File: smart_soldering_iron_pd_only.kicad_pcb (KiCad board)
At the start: 2 copper layers, 15 x 99.9 mm, 89 parts, among them J1 Conn_01x04_Pin, J2 TIP_SMALL_END, J3 TIP_MID, U3 ATMEGA328P-AU, U5 CH224K, Y1 16 MHZ

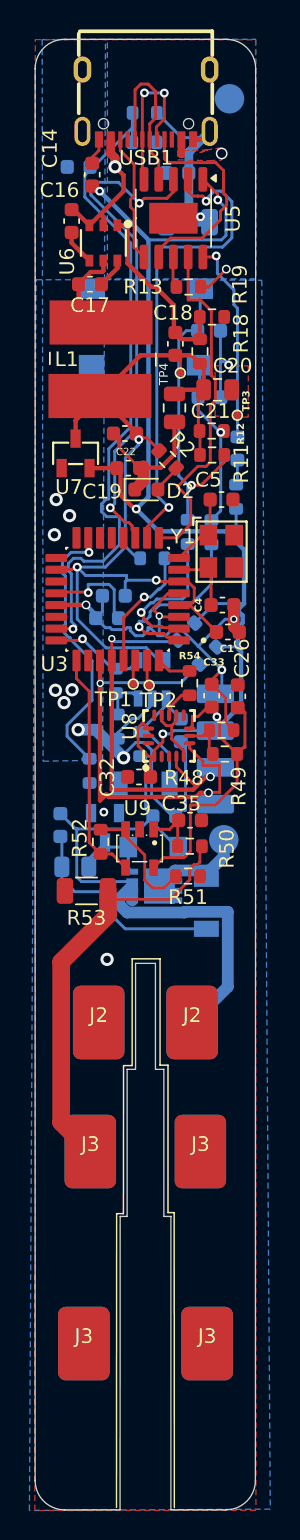
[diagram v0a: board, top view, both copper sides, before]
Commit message: added reset
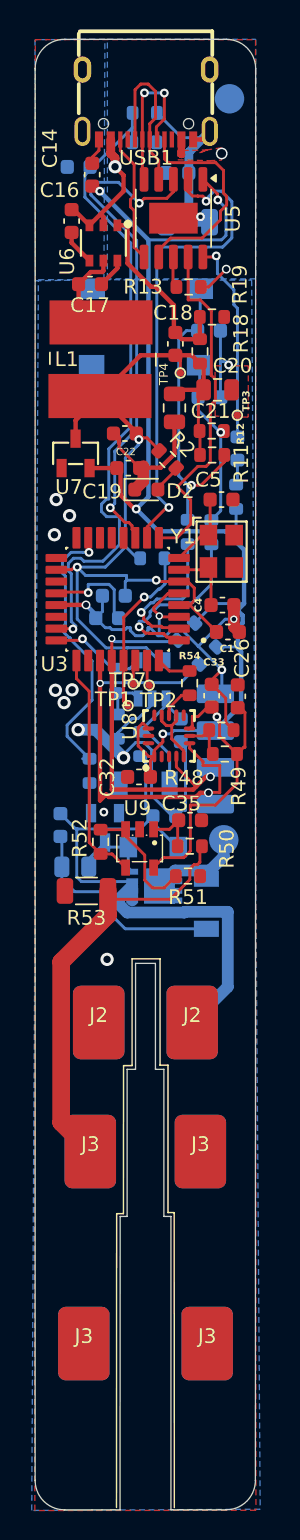
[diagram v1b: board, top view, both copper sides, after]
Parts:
- added TP7: TestPoint, TestPoint:TestPoint_Pad_D1.5mm, F.Cu at (191.3, 95.2)
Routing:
- net Net-(U3-PC6/~{RESET}): track 8.45 -> 11.6 mm
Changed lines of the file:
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@@
 	(footprint "TestPoint:TestPoint_Pad_D1.5mm"
 		(layer "F.Cu")
+		(at 191.3 95.21)
+		(descr "SMD pad as test Point, diameter 1.5mm")
+		(tags "test point SMD pad")
+		(property "Reference" "TP7"
+			(at 0 -1.648 0)
+			(layer "F.SilkS")
+			(effects
+				(font
+					(size 1 1)
+					(thickness 0.15)
+				)
+			)
+		)
+		(property "Value" "TestPoint"
+			(at 0 1.75 0)
+			(layer "F.Fab")
+			(hide yes)
+			(effects
+				(font
+					(size 1 1)
+					(thickness 0.15)
+				)
+			)
+		)
+		(property "Datasheet" "~"
+			(at 0 0 0)
+			(unlocked yes)
+			(layer "F.Fab")
+			(hide yes)
+			(effects
+				(font
+					(size 1.27 1.27)
+					(thickness 0.15)
+				)
+			)
+		)
+		(property "Description" "test point"
+			(at 0 0 0)
+			(unlocked yes)
+			(layer "F.Fab")
+			(hide yes)
+			(effects
+				(font
+					(size 1.27 1.27)
+					(thickness 0.15)
+				)
+			)
+		)
+		(property ki_fp_filters "Pin* Test*")
+		(sheetname "/")
+		(sheetfile "smart_soldering_iron_pd_only.kicad_sch")
+		(attr exclude_from_pos_files)
+		(fp_circle
+			(center 0.01 0.08)
+			(end 0.34 0.06)
+			(stroke
+				(width 0.12)
+				(type solid)
+			)
+			(fill no)
+			(layer "F.SilkS")
+		)
+		(fp_circle
+			(center 0.01 0.08)
+			(end 0.43 0)
+			(stroke
+				(width 0.05)
+				(type solid)
+			)
+			(fill no)
+			(layer "F.CrtYd")
+		)
+		(pad "1" smd circle
+			(at 0.01 0.08)
+			(size 0.5 0.5)
+			(layers "F.Cu" "F.Mask")
+			(net 62 "Net-(U3-PC6{slash}~{RESET})")
+			(pinfunction "1")
+			(pintype "passive")
+		)
+		(embedded_fonts no)
+	)
+	(footprint "TestPoint:TestPoint_Pad_D1.5mm"
+		(layer "F.Cu")
 		(at 191.66 93.74)
 		(descr "SMD pad as test Point, diameter 1.5mm")
@@
 	)
 	(segment
+		(start 191.01 92.22)
+		(end 191.01 94.99)
+		(width 0.2)
+		(layer "F.Cu")
+		(net 62)
+	)
+	(segment
 		(start 192.41 87.9)
 		(end 191.02 89.29)
@@
 	)
 	(segment
+		(start 191.01 94.99)
+		(end 191.31 95.29)
+		(width 0.2)
+		(layer "F.Cu")
+		(net 62)
+	)
+	(segment
 		(start 191.02 89.29)
 		(end 191.02 92.21)
@@
 		(polygon
 			(pts
-				(xy 189.78164 50.002272) (xy 185.479488 50.022282) (xy 185.541094 99.060641) (xy 189.584587 98.99325)
+				(xy 189.741598 50.002459) (xy 184.990808 50.024555) (xy 185.011394 66.411142) (xy 189.675911 66.333401)
 			)
 		)
@@
 		(polygon
 			(pts
-				(xy 189.71 66.34) (xy 200.403147 66.373243) (xy 200.983085 149.894381) (xy 184.612682 149.982572)
-				(xy 185.06379 66.34)
+				(xy 189.71 66.34) (xy 199.715703 66.371106) (xy 200.295682 149.898084) (xy 184.769335 149.981728)
+				(xy 185.220439 66.34)
 			)
 		)
